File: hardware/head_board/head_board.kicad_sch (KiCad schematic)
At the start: 3 parts

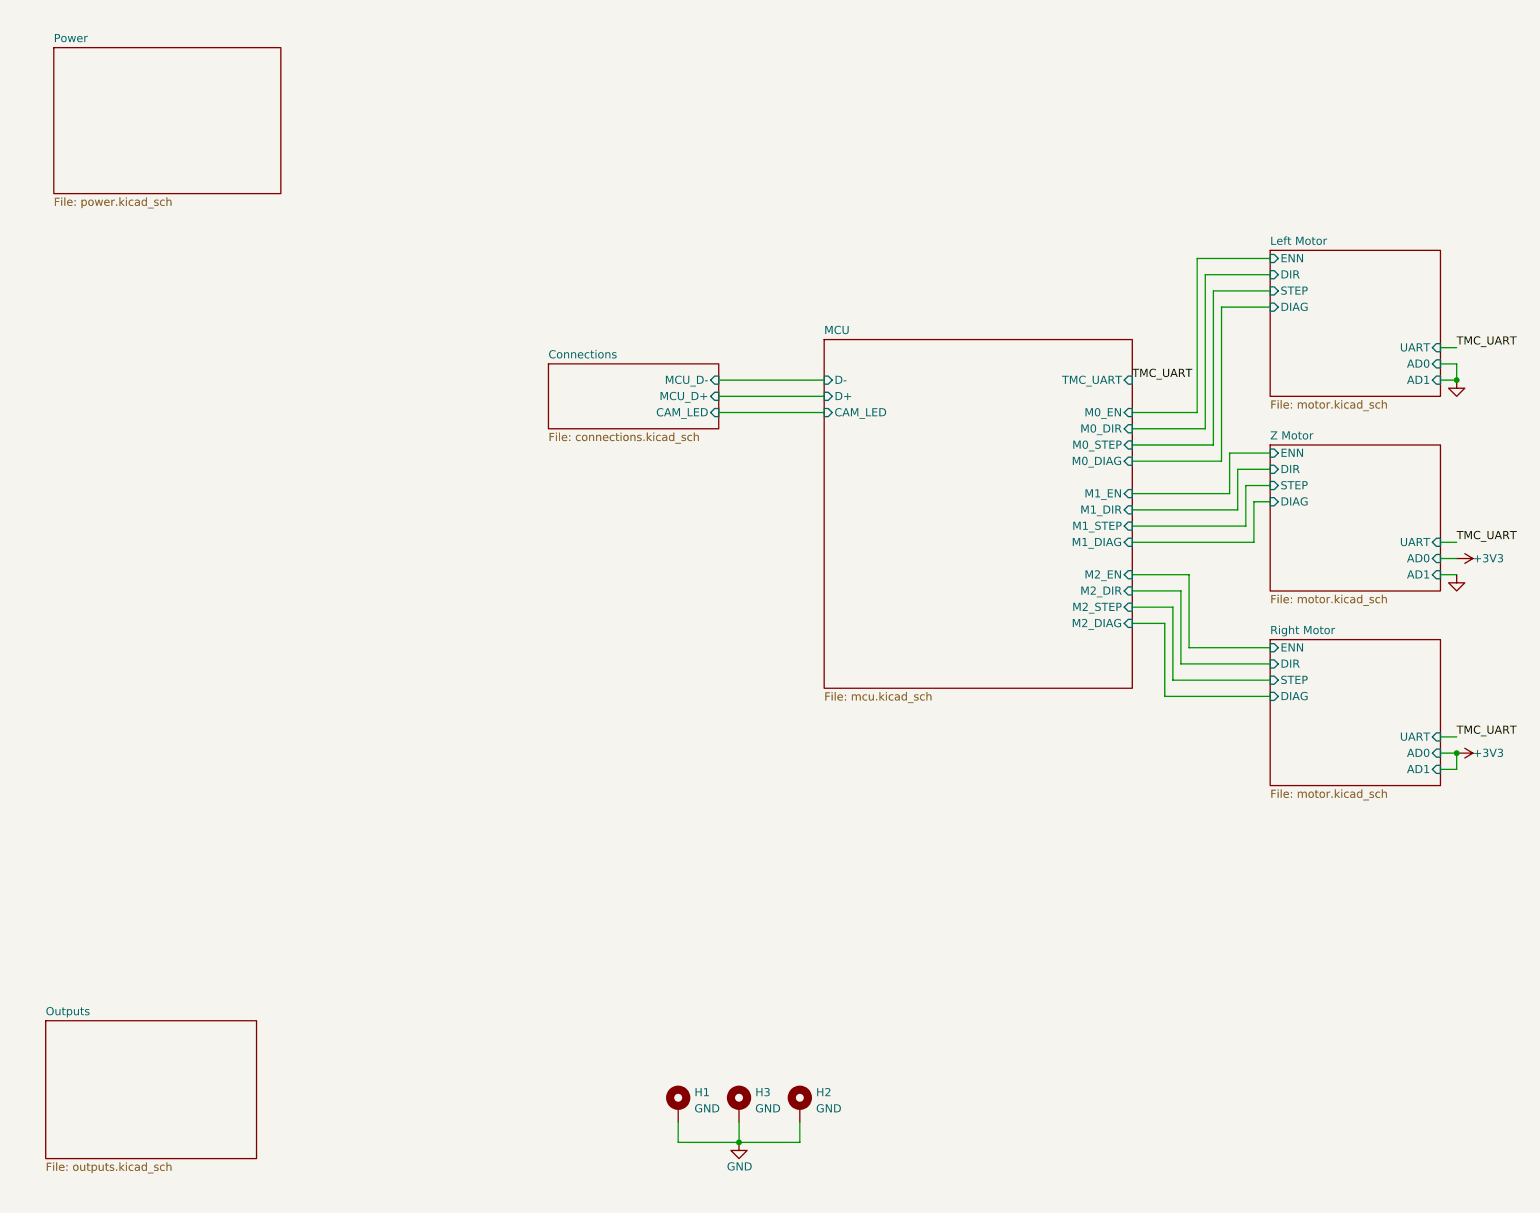
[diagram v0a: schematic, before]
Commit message: v1 revision to the schematic
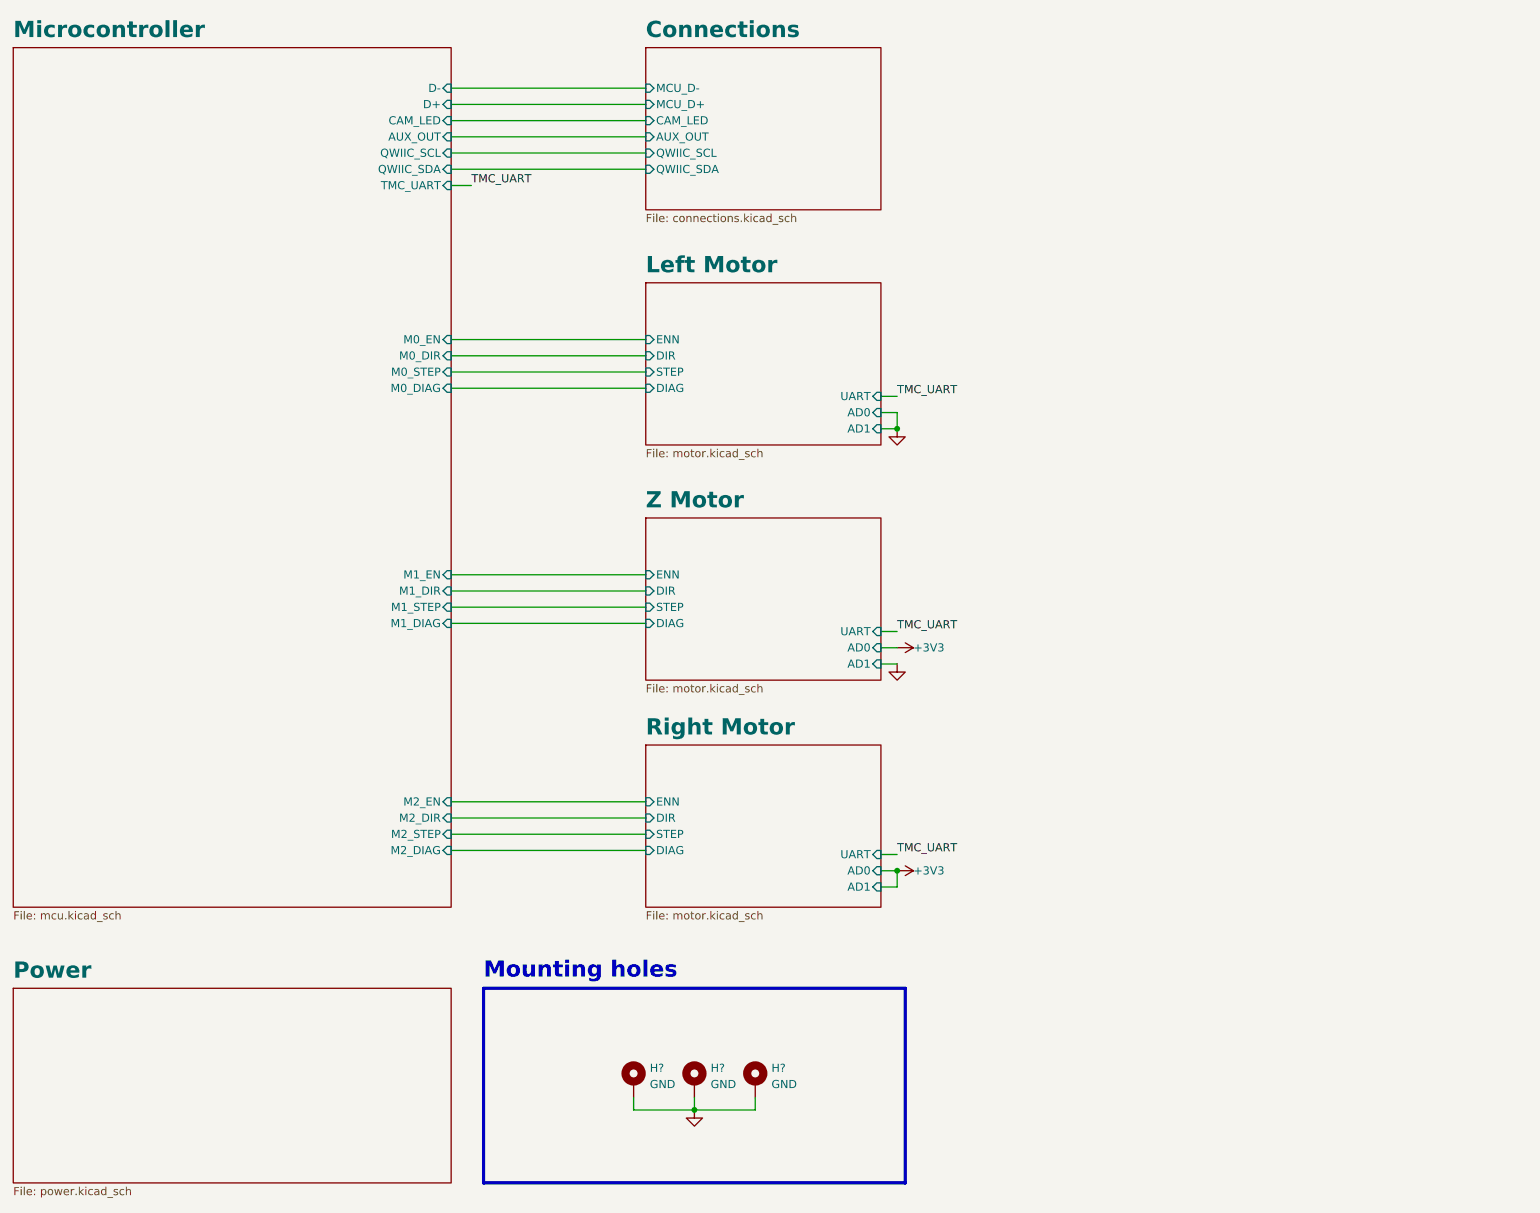
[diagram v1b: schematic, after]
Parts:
- removed H1, H2, H3: GND, MountingHole:MountingHole_3mm_Pad, symbol Mechanical:MountingHole_Pad
- added H? (x3): GND, MountingHole:MountingHole_3mm_Pad, symbol Mechanical:MountingHole_Pad
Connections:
- net GND: now also H?.1, H?.1, H?.1
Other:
- sheet MCU renamed Microcontroller
- removed sheet Outputs
- sheet Connections ports: added AUX_OUT, QWIIC_SCL, QWIIC_SDA; removed none
- sheet Microcontroller ports: added AUX_OUT, QWIIC_SCL, QWIIC_SDA; removed none
- note added: "Mounting holes"
- title: Candela (head) -> Candela Head
